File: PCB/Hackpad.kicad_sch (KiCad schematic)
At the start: 21 parts, among them J1 OLED_128x64, SW1 RotaryEncoder_Switch, U1 MCU_Seeed_XIAO_RP2040

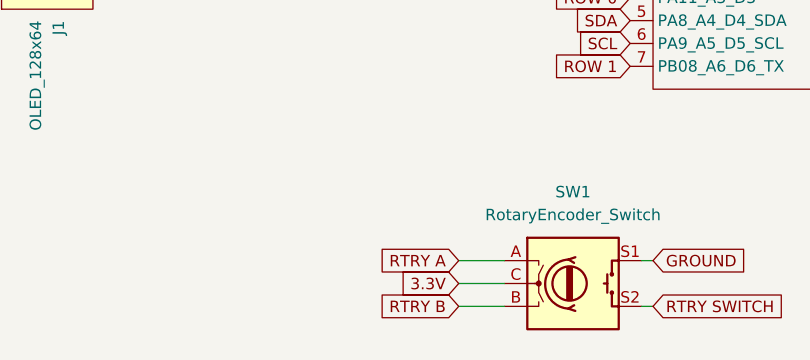
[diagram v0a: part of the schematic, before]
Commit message: Updated Image Files v3
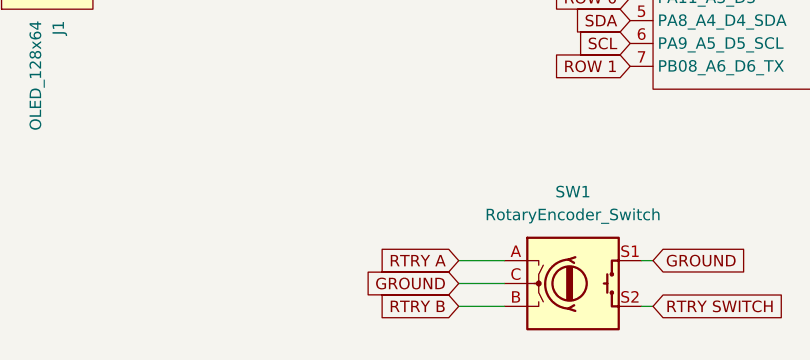
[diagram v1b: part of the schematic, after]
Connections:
- net 3.3V: no longer SW1.C
- net GROUND: now also SW1.C
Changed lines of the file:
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@@
 		)
 	)
-	(global_label "3.3V"
+	(global_label "GROUND"
 		(shape input)
 		(at 69.85 72.39 180)
@@
 		)
 		(property "Intersheetrefs" "${INTERSHEET_REFS}"
-			(at 62.7524 72.39 0)
+			(at 59.0633 72.39 0)
 			(effects
 				(font
